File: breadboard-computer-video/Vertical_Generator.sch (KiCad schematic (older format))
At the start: 7 parts, among them U1 74LS04, U10 74LS08, U11 74LS02, U12 74LS163, U13 74LS04, U14 74LS30, U15 74LS163

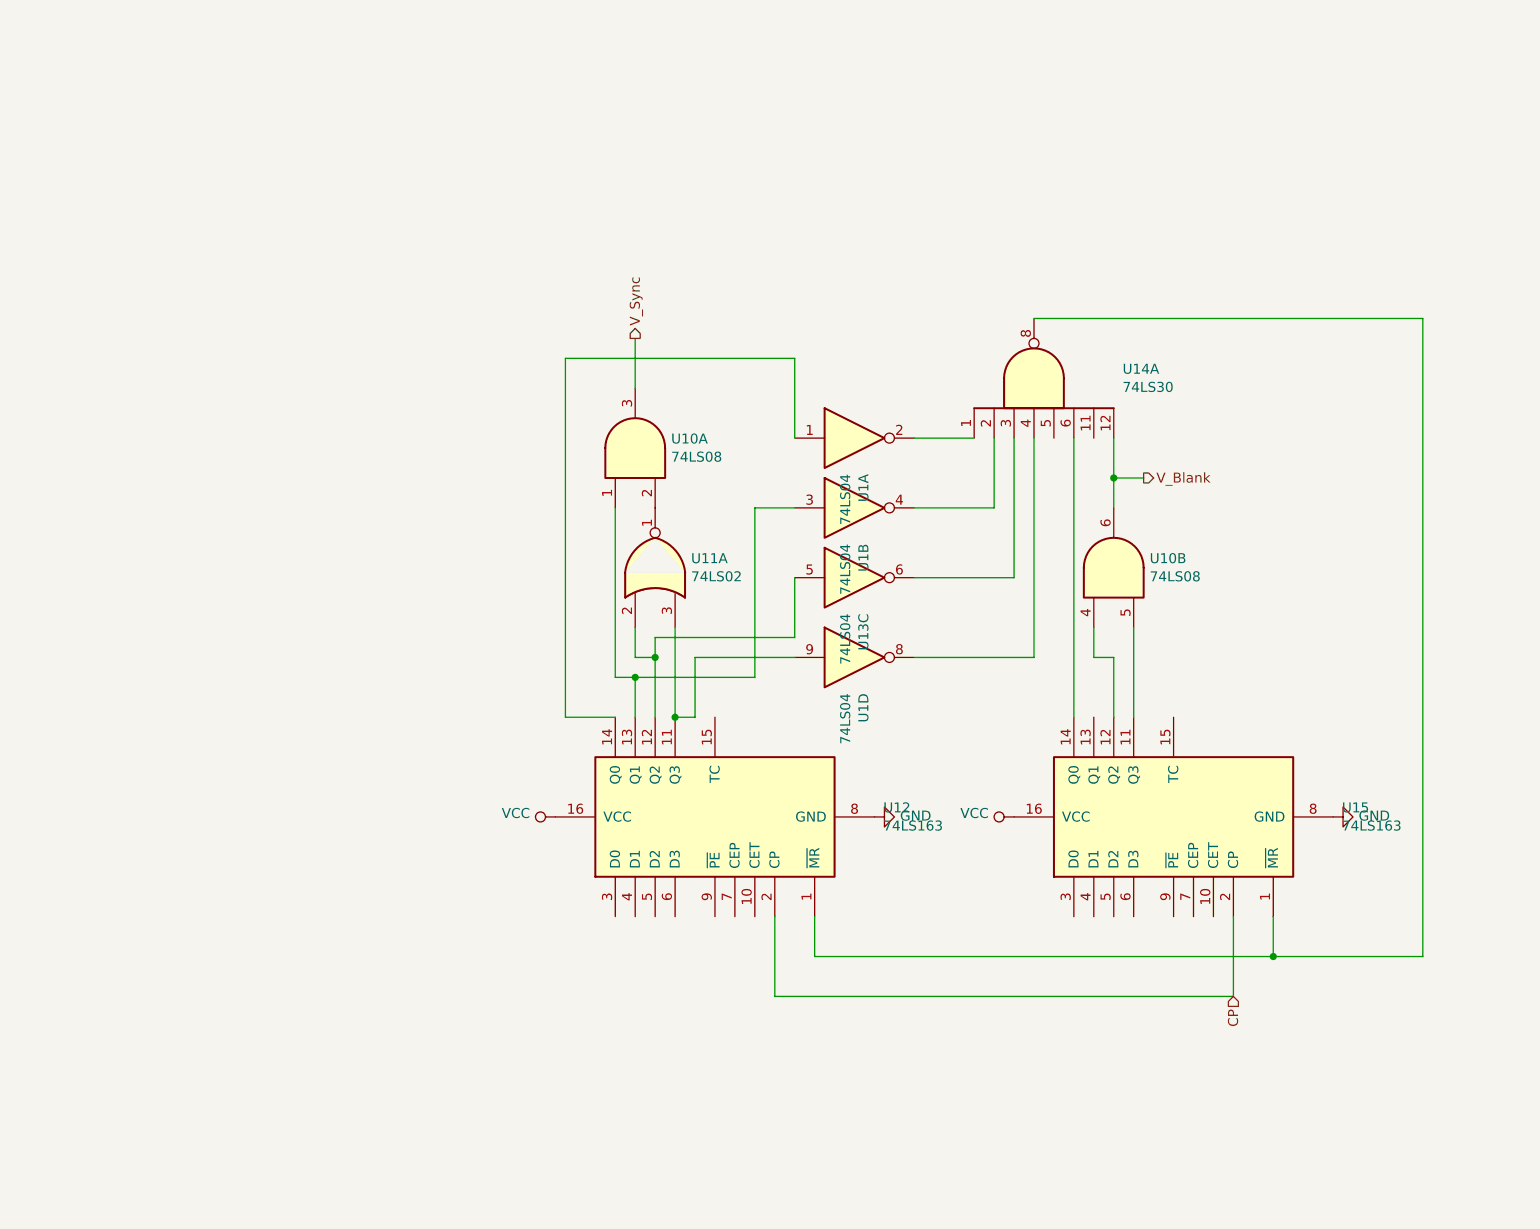
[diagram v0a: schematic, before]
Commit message: finished hv sync
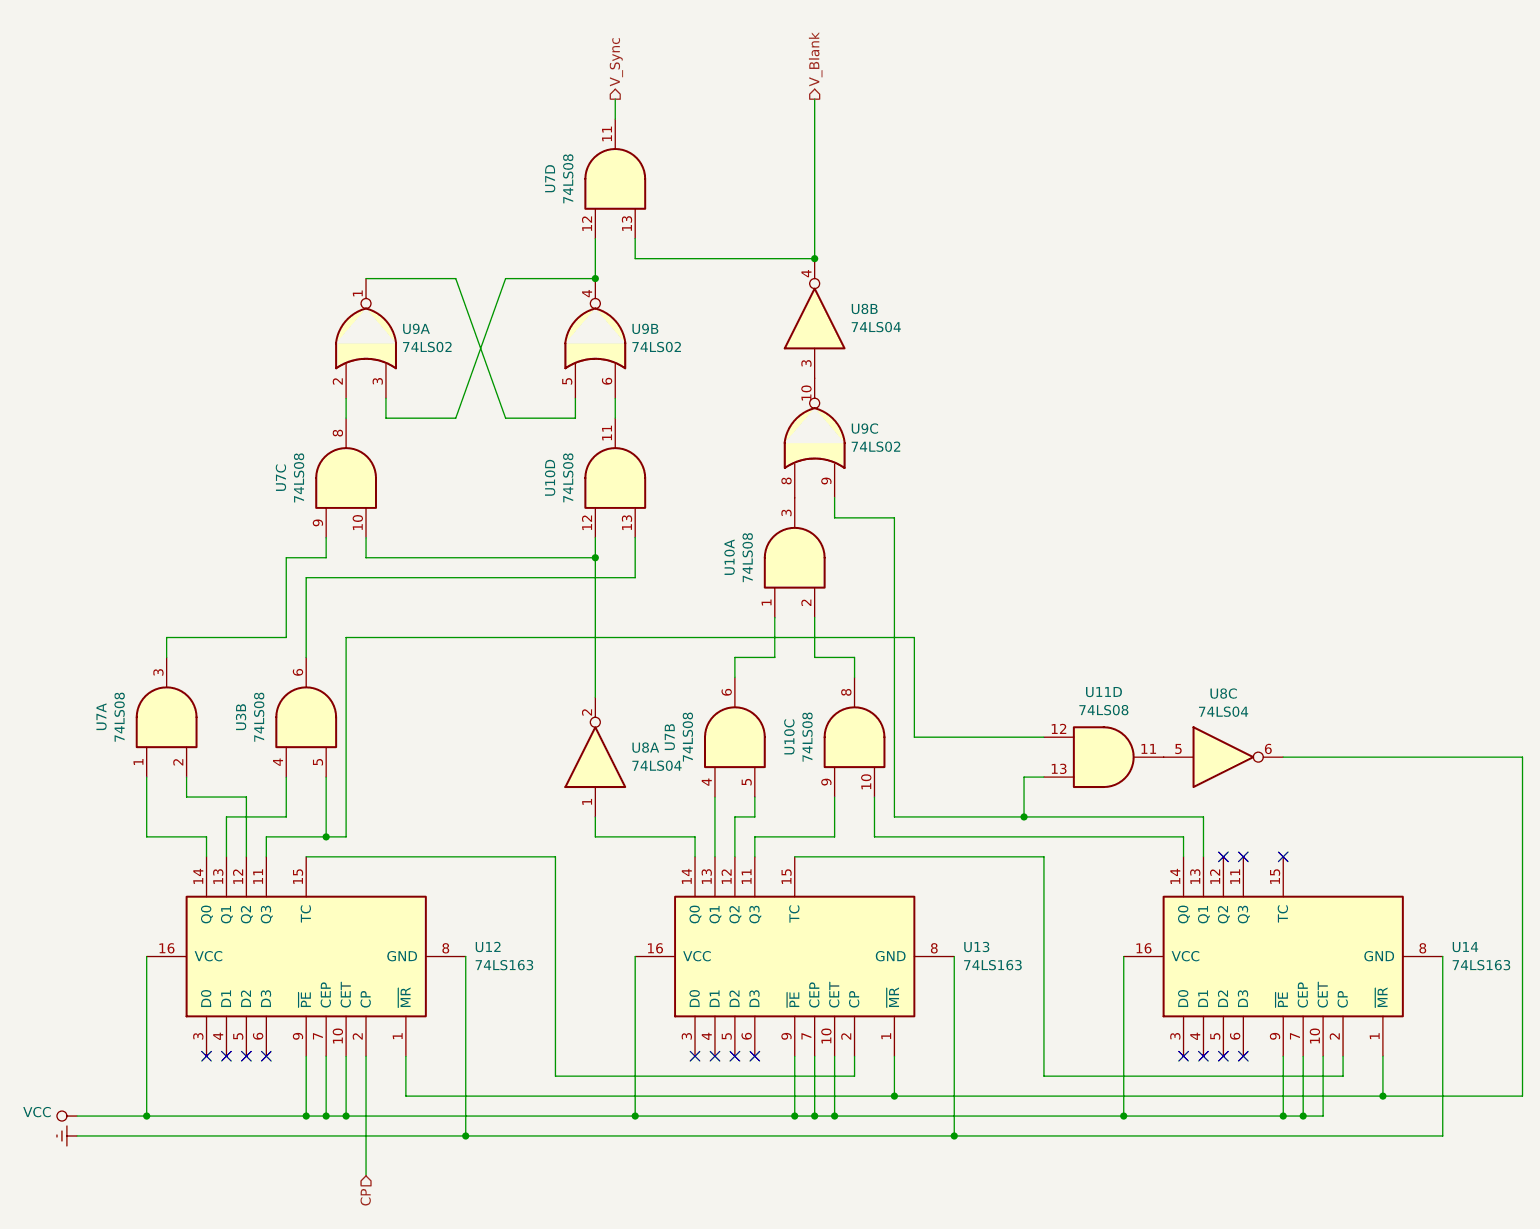
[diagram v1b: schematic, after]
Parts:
- removed U1, U13: 74LS04, symbol 74xx:74LS04
- removed unit 2 of U10
- removed U11: 74LS02, symbol 74xx:74LS02
- removed U14: 74LS30, symbol 74xx:74LS30
- added unit 3 of U10
- added unit 4 of U10
- added U11, U3, U7: 74LS08, symbol 74xx:74LS08
- added U14: 74LS163, symbol 74xx:74LS163
- added U8: 74LS04, symbol 74xx:74LS04
- added U9: 74LS02, symbol 74xx:74LS02
- renumbered U15 to U13
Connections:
- net CP: no longer U13.2 (CP)
- net VCC: now also U12.10 (CET), U12.7 (CEP), U12.9 (~PE), U13.10 (CET), U13.7 (CEP), U13.9 (~PE), U14.10 (CET), U14.16 (VCC), U14.7 (CEP), U14.9 (~PE)
- net V_Blank: now also U7.13, U8.4
- net V_Sync: now also U7.11; no longer U10.3
- net at U10.1: now also U7.6; no longer U12.13 (Q1)
- net at U10.2: now also U10.8
- net at U12.12 (Q2): now also U7.2
- net at U12.11 (Q3): now also U11.12, U3.5
- net at U13.14 (Q0): now also U8.1
- net at U12.1 (~MR), U13.1 (~MR): now also U14.1 (~MR), U8.6
- net at U12.14 (Q0): now also U7.1
- net at U13.12 (Q2): now also U7.5
- net at U13.11 (Q3): now also U10.9
- net at U12.15 (TC): now also U13.2 (CP)
- net at U13.13 (Q1): now also U7.4
- net at U13.15 (TC): now also U14.2 (CP)
- net GND renamed Earth
- net Earth: now also U14.8 (GND)
- new net: U9.1, U9.5
- new net: U7.8, U9.2
- new net: U7.12, U9.3, U9.4
- new net: U10.11, U9.6
- new net: U8.3, U9.10
- new net: U10.3, U9.8
- new net: U11.13, U14.13 (Q1), U9.9
- new net: U10.10, U14.14 (Q0)
- new net: U10.12, U7.10, U8.2
- new net: U10.13, U3.6
- new net: U7.3, U7.9
- new net: U12.13 (Q1), U3.4
- new net: U11.11, U8.5
- no-connect marks 0 -> 15
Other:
- moved on the sheet: U12, U13
